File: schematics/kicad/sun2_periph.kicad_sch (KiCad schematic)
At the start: 2 parts, among them U610 74LS04, U613 74LS05

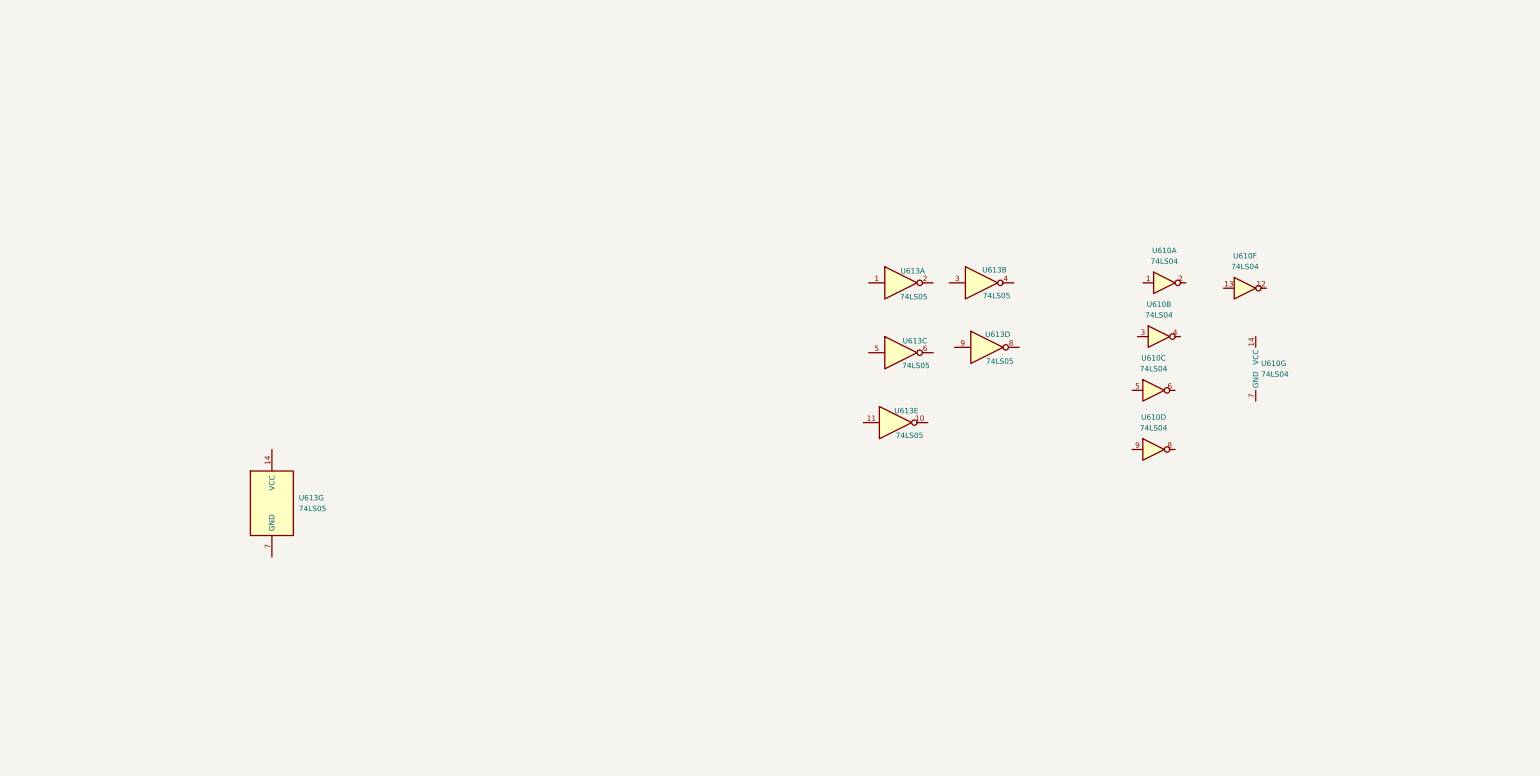
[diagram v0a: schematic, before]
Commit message: Serials
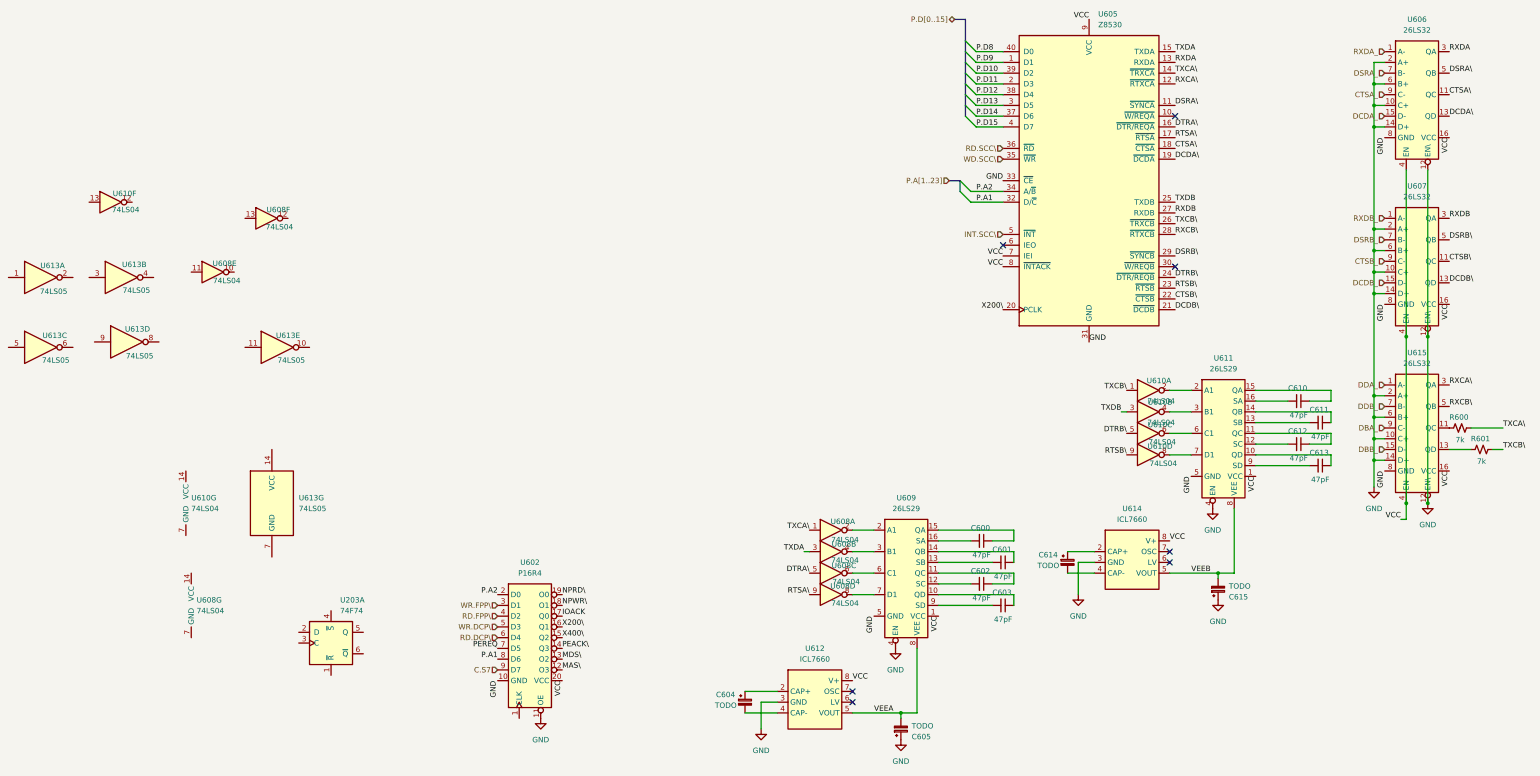
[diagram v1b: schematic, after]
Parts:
- added C600, C601, C602, C603, C610, C611, C612, C613: 47pF, symbol Device:C_Small
- added C604, C605, C614, C615: TODO, symbol Device:C_Polarized_Small
- added R600, R601: 7k, symbol Device:R_Small_US
- added U203: 74F74, Package_DIP:DIP-14_W7.62mm, symbol sun2:74F74
- added U602: P16R4, Package_DIP:DIP-20_W7.62mm, symbol sun2:P16R4
- added U605: Z8530, Package_DIP:DIP-40_W15.24mm, symbol Interface_UART:Z8530
- added U606, U607, U615: 26LS32, Package_DIP:DIP-16_W7.62mm, symbol sun2:26LS32
- added U608: 74LS04, Package_DIP:DIP-14_W7.62mm, symbol sun2:74LS04
- added U609, U611: 26LS29, Package_DIP:DIP-16_W7.62mm, symbol sun2:26LS29
- added U612, U614: ICL7660, Package_DIP:DIP-8_W7.62mm, symbol sun2:ICL7660
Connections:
- net TXDB: now reaches U610.3
- net TXDB: now also U605.25 (TXDB)
- net at U610.4: now also U611.3 (B1)
- net DTRB\: now reaches U610.5
- net DTRB\: now also U605.24 (~{DTR/REQB})
- net at U610.6: now also U611.6 (C1)
- net TXCB\: now reaches U610.1
- net TXCB\: now also R601.2, U605.26 (~{TRXCB})
- net at U610.2: now also U611.2 (A1)
- net at U610.8: now also U611.7 (D1)
- net RTSB\: now reaches U610.9
- net RTSB\: now also U605.23 (~{RTSB})
- new net: C614.1, U614.2 (CAP+)
- new net: C614.2, U614.4 (CAP-)
- new net: U608.2, U609.2 (A1)
- new net: C613.1, U611.10 (QD)
- new net: C613.2, U611.9 (SD)
- new net: C601.1, U609.14 (QB)
- new net: C601.2, U609.13 (SB)
- new net: U608.6, U609.6 (C1)
- new net: R600.1, U615.11 (QC)
- new net: C603.1, U609.10 (QD)
- new net: C602.1, U609.11 (QC)
- new net: C602.2, U609.12 (SC)
- new net: C600.1, U609.15 (QA)
- new net: C600.2, U609.16 (SA)
- new net: U608.4, U609.3 (B1)
- new net: U608.8, U609.7 (D1)
- new net: C603.2, U609.9 (SD)
- new net: C604.1, U612.2 (CAP+)
- new net: C604.2, U612.4 (CAP-)
- new net: C610.1, U611.15 (QA)
- new net: C610.2, U611.16 (SA)
- new net: C612.1, U611.11 (QC)
- new net: C612.2, U611.12 (SC)
- new net: C611.1, U611.14 (QB)
- new net: C611.2, U611.13 (SB)
- new net: R601.1, U615.13 (QD)
- new net C.S7: U602.9 (D7)
- new net CTSA\: U605.18 (~{CTSA}), U606.11 (QC)
- new net CTSA_: U606.9 (C-)
- new net CTSB\: U605.22 (~{CTSB}), U607.11 (QC)
- new net CTSB_: U607.9 (C-)
- new net DBA_: U615.9 (C-)
- new net DBB_: U615.15 (D-)
- new net DCDA\: U605.19 (~{DCDA}), U606.13 (QD)
- new net DCDA_: U606.15 (D-)
- new net DCDB\: U605.21 (~{DCDB}), U607.13 (QD)
- new net DCDB_: U607.15 (D-)
- new net DDA_: U615.1 (A-)
- new net DDB_: U615.7 (B-)
- new net DSRA\: U605.11 (~{SYNCA}), U606.5 (QB)
- new net DSRA_: U606.7 (B-)
- new net DSRB\: U605.29 (~{SYNCB}), U607.5 (QB)
- new net DSRB_: U607.7 (B-)
- new net DTRA\: U605.16 (~{DTR/REQA}), U608.5
- new net GND: C605.1, C615.1, U602.10 (GND), U602.11 (OE), U605.31 (GND), U605.33 (~{CE}), U606.10 (C+), U606.12 (EN\), U606.14 (D+), U606.2 (A+), U606.6 (B+), U606.8 (GND), U607.10 (C+), U607.12 (EN\), U607.14 (D+), U607.2 (A+), U607.6 (B+), U607.8 (GND), U609.4 (EN), U609.5 (GND), U611.4 (EN), U611.5 (GND), U612.3 (GND), U614.3 (GND), U615.10 (C+), U615.12 (EN\), U615.14 (D+), U615.2 (A+), U615.6 (B+), U615.8 (GND)
- new net INT.SCC\: U605.5 (~{INT})
- new net IOACK: U602.17 (Q0)
- new net MAS\: U602.12 (O3)
- new net MDS\: U602.13 (O2)
- new net NPRD\: U602.19 (O0)
- new net NPWR\: U602.18 (O1)
- new net P.A1: U602.8 (D6), U605.32 (D/~{C})
- new net P.A2: U602.2 (D0), U605.34 (A/~{B})
- new net P.D10: U605.39 (D2)
- new net P.D11: U605.2 (D3)
- new net P.D12: U605.38 (D4)
- new net P.D13: U605.3 (D5)
- new net P.D14: U605.37 (D6)
- new net P.D15: U605.4 (D7)
- new net P.D8: U605.40 (D0)
- new net P.D9: U605.1 (D1)
- new net PEACK\: U602.14 (Q3)
- new net PEREQ: U602.7 (D5)
- new net RD.DCP\: U602.6 (D4)
- new net RD.FPP\: U602.4 (D2)
- new net RD.SCC\: U605.36 (~{RD})
- new net RTSA\: U605.17 (~{RTSA}), U608.9
- new net RXCA\: U605.12 (~{RTXCA}), U615.3 (QA)
- new net RXCB\: U605.28 (~{RTXCB}), U615.5 (QB)
- new net RXDA: U605.13 (RXDA), U606.3 (QA)
- new net RXDA_: U606.1 (A-)
- new net RXDB: U605.27 (RXDB), U607.3 (QA)
- new net RXDB_: U607.1 (A-)
- new net TXCA\: R600.2, U605.14 (~{TRXCA}), U608.1
- new net TXDA: U605.15 (TXDA), U608.3
- new net VCC: U602.20 (VCC), U605.7 (IEI), U605.8 (~{INTACK}), U605.9 (VCC), U606.16 (VCC), U606.4 (EN), U607.16 (VCC), U607.4 (EN), U609.1 (VCC), U611.1 (VCC), U612.8 (V+), U614.8 (V+), U615.16 (VCC), U615.4 (EN)
- new net VEEA: C605.2, U609.8 (VEE), U612.5 (VOUT)
- new net VEEB: C615.2, U611.8 (VEE), U614.5 (VOUT)
- new net WD.SCC\: U605.35 (~{WR})
- new net WR.DCP\: U602.5 (D3)
- new net WR.FPP\: U602.3 (D1)
- new net X200\: U602.16 (Q1), U605.20 (PCLK)
- new net X400\: U602.15 (Q2)
- no-connect marks 0 -> 7
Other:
- moved on the sheet: U610A, U610B, U610C, U610D, U610F, U610G, U613A, U613B, U613C, U613D, U613E

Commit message: Timer
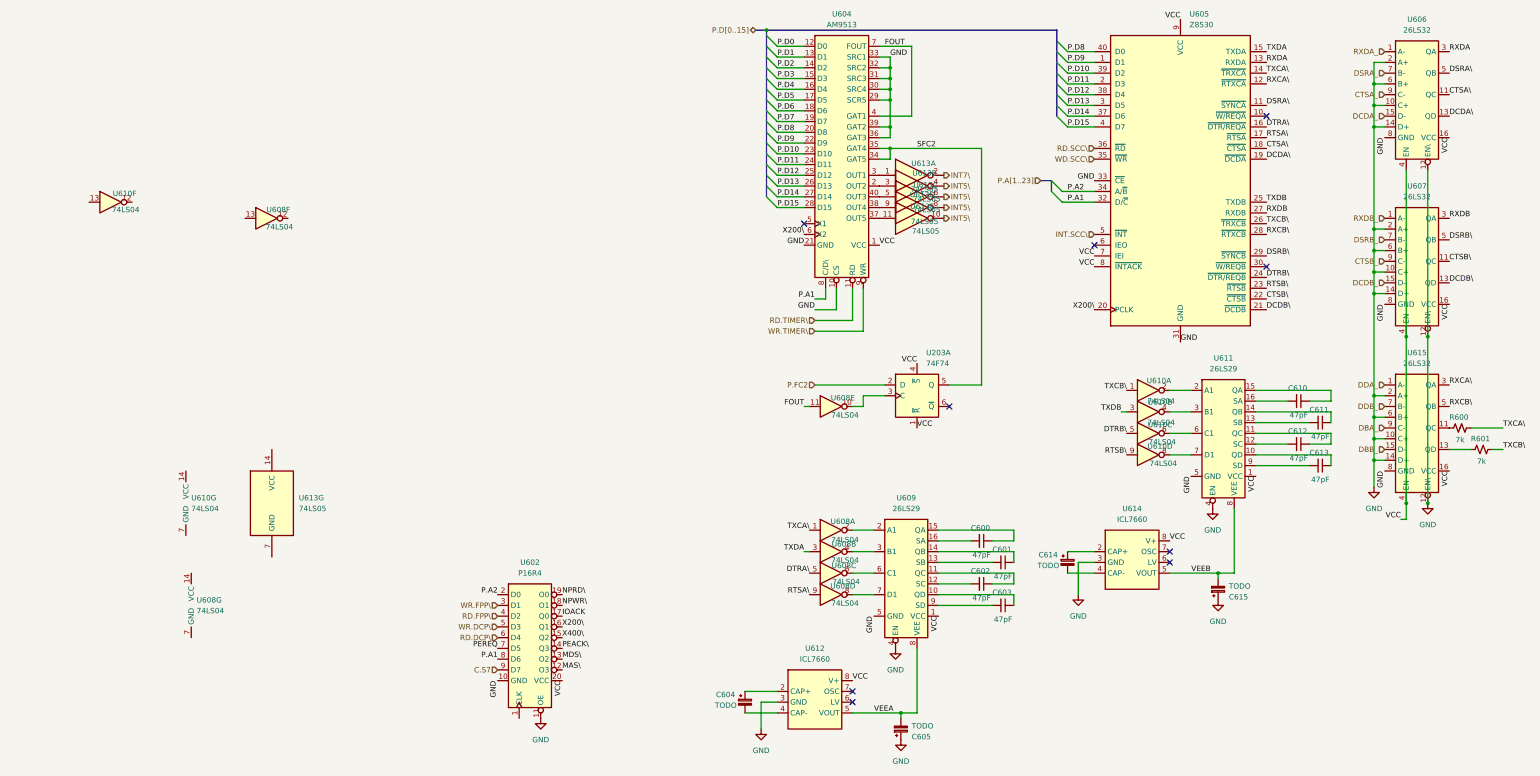
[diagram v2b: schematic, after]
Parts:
- added U604: AM9513, Package_DIP:DIP-40_W15.24mm, symbol sun2:AM9513
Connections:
- net GND: now also U604.10 (CS), U604.21 (GND), U604.29 (SCR5), U604.30 (SRC4), U604.31 (SRC3), U604.32 (SRC2), U604.33 (SRC1), U604.36 (GAT3), U604.39 (GAT2)
- net P.A1: now also U604.8 (C/D\)
- net P.D10: now also U604.23 (D10)
- net P.D11: now also U604.24 (D11)
- net P.D12: now also U604.25 (D12)
- net P.D13: now also U604.26 (D13)
- net P.D14: now also U604.27 (D14)
- net P.D15: now also U604.28 (D15)
- net P.D8: now also U604.20 (D8)
- net P.D9: now also U604.22 (D9)
- net VCC: now also U203.1 (~{R}), U203.4 (~{S}), U604.1 (VCC)
- net X200\: now also U604.6 (X2)
- net at U613.3: now also U604.2 (OUT2)
- net INT5\: now reaches U613.4
- net INT5\: now also U613.10, U613.6, U613.8
- net at U613.11: now also U604.37 (OUT5)
- net at U613.1: now also U604.3 (OUT1)
- net INT7\: now reaches U613.2
- net at U613.5: now also U604.40 (OUT3)
- net at U613.9: now also U604.38 (OUT4)
- net at U608.10: now also U203.3 (C)
- net FOUT: now reaches U608.11
- net FOUT: now also U604.4 (GAT1), U604.7 (FOUT)
- net P.FC2: now reaches U203.2 (D)
- net SFC2: now reaches U203.5 (Q)
- net SFC2: now also U604.34 (GAT5), U604.35 (GAT4)
- new net P.D0: U604.12 (D0)
- new net P.D1: U604.13 (D1)
- new net P.D2: U604.14 (D2)
- new net P.D3: U604.15 (D3)
- new net P.D4: U604.16 (D4)
- new net P.D5: U604.17 (D5)
- new net P.D6: U604.18 (D6)
- new net P.D7: U604.19 (D7)
- new net RD.TIMER\: U604.11 (RD)
- new net WR.TIMER\: U604.9 (WR)
- no-connect marks 7 -> 9
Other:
- moved on the sheet: U203A, U605, U608E, U613A, U613B, U613C, U613D, U613E
